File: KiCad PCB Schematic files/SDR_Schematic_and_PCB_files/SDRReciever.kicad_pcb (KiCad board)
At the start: 2 copper layers, 83 x 34.7 mm, 66 parts, among them J1 Conn_Coaxial, J10 I_0, J11 I_180, J12 Q_90, J13 Q_270, J14 AudioJack3, J2 3.3V, J3 FIL_IN, J4 5V, J5 4.3V, J6 FIL_OUT, J7 CLK_2, J8 CLK_0, J9 CLK_1, Q1 MMBT2222A-TP, Q2 BSS138, Q3 BSS138, U1 Si5351A-B-GT, U2 SN74CBT3253, U3 LM4562, Y1 CX3225SB

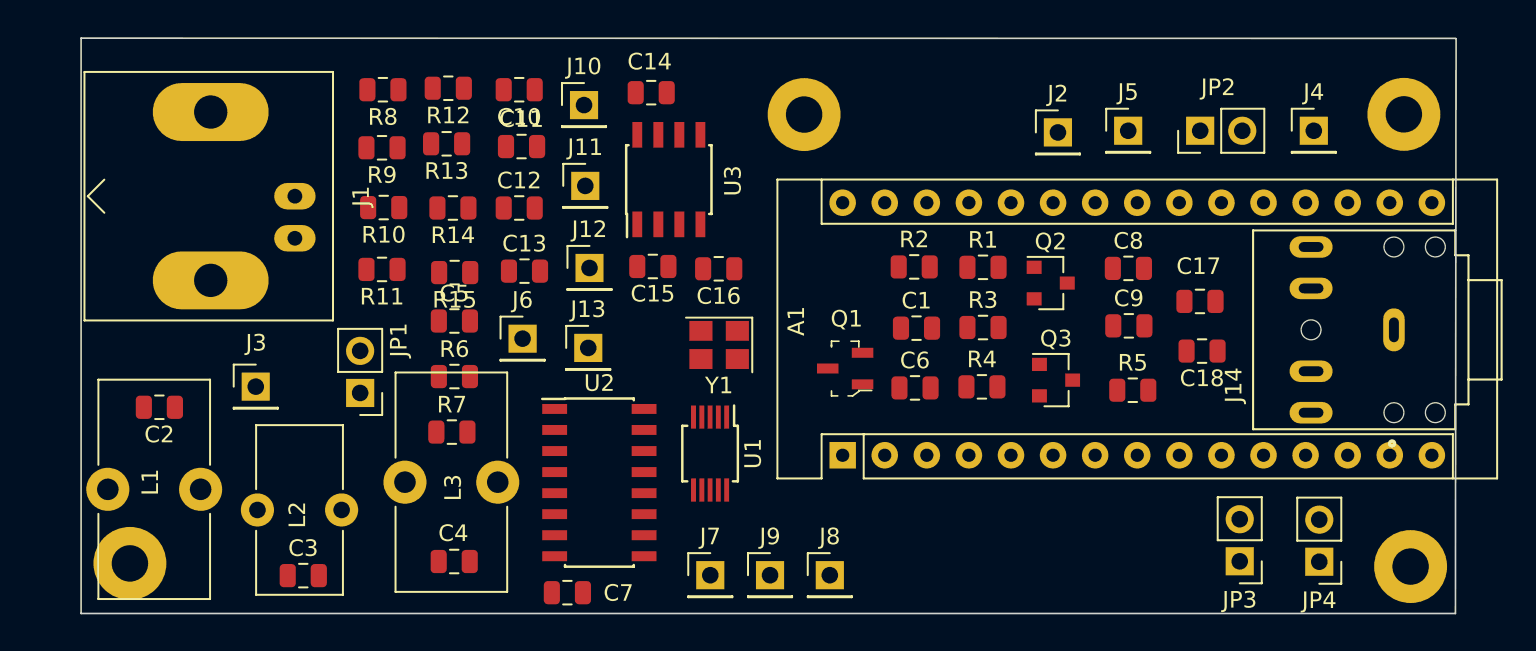
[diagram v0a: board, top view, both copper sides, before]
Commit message: Revised PCB part placement
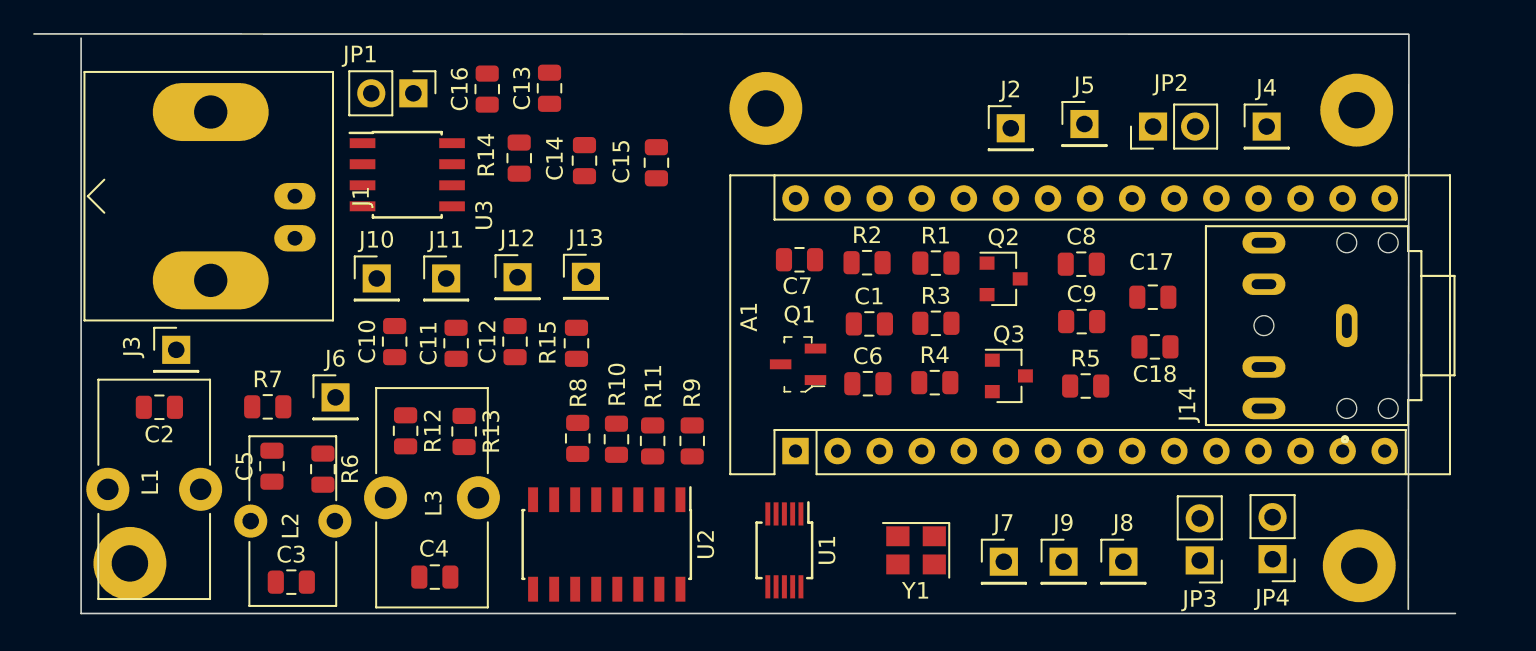
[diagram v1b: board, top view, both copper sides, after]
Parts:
- moved R9 25.8 mm to (133.4, 139.4), turned to 270 degrees
- moved C7 24.5 mm to (139.9, 128.5), turned to 0 degrees
- moved R8 24.1 mm to (126.5, 139.2), turned to 270 degrees
- moved R12 20.8 mm to (116.1, 138.8), turned to 270 degrees
- moved R10 19.8 mm to (128.9, 139.3), turned to 270 degrees
- moved R11 19.3 mm to (131.0, 139.4), turned to 270 degrees
- moved JP1 18.4 mm to (116.6, 118.4), turned to 270 degrees
- moved J7 17.7 mm to (152.2, 146.7)
- moved J8 17.7 mm to (159.4, 146.7)
- moved J9 17.7 mm to (155.8, 146.7)
- moved C16 17.7 mm to (121.1, 118.2), turned to 90 degrees
- moved R13 17.4 mm to (119.7, 138.8), turned to 270 degrees
- moved Y1 17.2 mm to (146.9, 146.0)
- moved C10 17.0 mm to (115.5, 133.4), turned to 90 degrees
- moved J10 16.3 mm to (114.4, 129.6)
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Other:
- board size 83 x 34.7 mm -> 85.8 x 35 mm
